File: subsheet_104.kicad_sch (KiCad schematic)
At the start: 0 parts

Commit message: almost done dma controller and acsi port
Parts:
- added C7: 0.1uF, commons-passives_THT:Passive_THT_capacitor_mlcc_W2.54mm_L12.70mm, symbol Device:C_Small
- added J2: DB19S ACSI, symbol Connector_Generic_Shielded:Conn_01x19_Shielded
- added L24: Ferrite bead, commons-passives_THT:Passive_THT_ferrite_bead_W3.81mm_L15.24mm, symbol Device:Ferrite_Bead_Small
- added R103: 1K, symbol Device:R_Small_US
- added U1: ST_DMA_DIP40_PHY, Package_DIP:DIP-40_W15.24mm_LongPads, symbol st_dma_dip40:ST_DMA_DIP40_PHY
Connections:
- new net +5V: L24.2, R103.2
- new net +5VP: C7.1, L24.1, U1.40 (VCC)
- new net 8MHZ: U1.39 (CLK)
- new net A1: U1.2 (A1)
- new net ACK: J2.14 (Pin_14), U1.37 (~{ACK})
- new net ACSI_PORT_DRQ: J2.19 (Pin_19), R103.1
- new net ACSI_PORT_INT: J2.10 (Pin_10)
- new net CA1: J2.16 (Pin_16), U1.26 (CA1)
- new net CA2: U1.27 (CA2)
- new net CD0: J2.1 (Pin_1), U1.36 (CD0)
- new net CD1: J2.2 (Pin_2), U1.35 (CD1)
- new net CD2: J2.3 (Pin_3), U1.34 (CD2)
- new net CD3: J2.4 (Pin_4), U1.33 (CD3)
- new net CD4: J2.5 (Pin_5), U1.32 (CD4)
- new net CD5: J2.6 (Pin_6), U1.31 (CD5)
- new net CD6: J2.7 (Pin_7), U1.30 (CD6)
- new net CD7: J2.8 (Pin_8), U1.29 (CD7)
- new net CS: J2.9 (Pin_9), U1.24 (~{HDCS})
- new net D0: U1.4 (D0)
- new net D1: U1.5 (D1)
- new net D10: U1.14 (D10)
- new net D11: U1.15 (D11)
- new net D12: U1.16 (D12)
- new net D13: U1.17 (D13)
- new net D14: U1.18 (D14)
- new net D15: U1.19 (D15)
- new net D2: U1.6 (D2)
- new net D3: U1.7 (D3)
- new net D4: U1.8 (D4)
- new net D5: U1.9 (D5)
- new net D6: U1.10 (D6)
- new net D7: U1.11 (D7)
- new net D8: U1.12 (D8)
- new net D9: U1.13 (D9)
- new net DMA_FDCS: U1.22 (~{FDCS})
- new net DMA_FDRQ: U1.21 (FDRQ)
- new net DMA_RW: J2.18 (Pin_18), U1.25 (CR/~{W})
- new net GND: C7.2, J2.11 (Pin_11), J2.13 (Pin_13), J2.15 (Pin_15), J2.17 (Pin_17), J2.SH (Shield), U1.20 (GND), U1.28 (GND)
- new net XFCS: U1.3 (~{FCS})
- new net XRDY: U1.38 (RDY)
- new net XRESET: J2.12 (Pin_12)
- new net XRXW: U1.1 (R/~{W})
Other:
- note added: "A1"
- note added: "D0"
- note added: "D1"
- note added: "D2"
- note added: "D3"
- note added: "D4"
- note added: "D5"
- note added: "D6"
- note added: "D7"
- note added: "DRQ"
- note added: "INT"
- note added: "R /W"
- note added: "RESET"

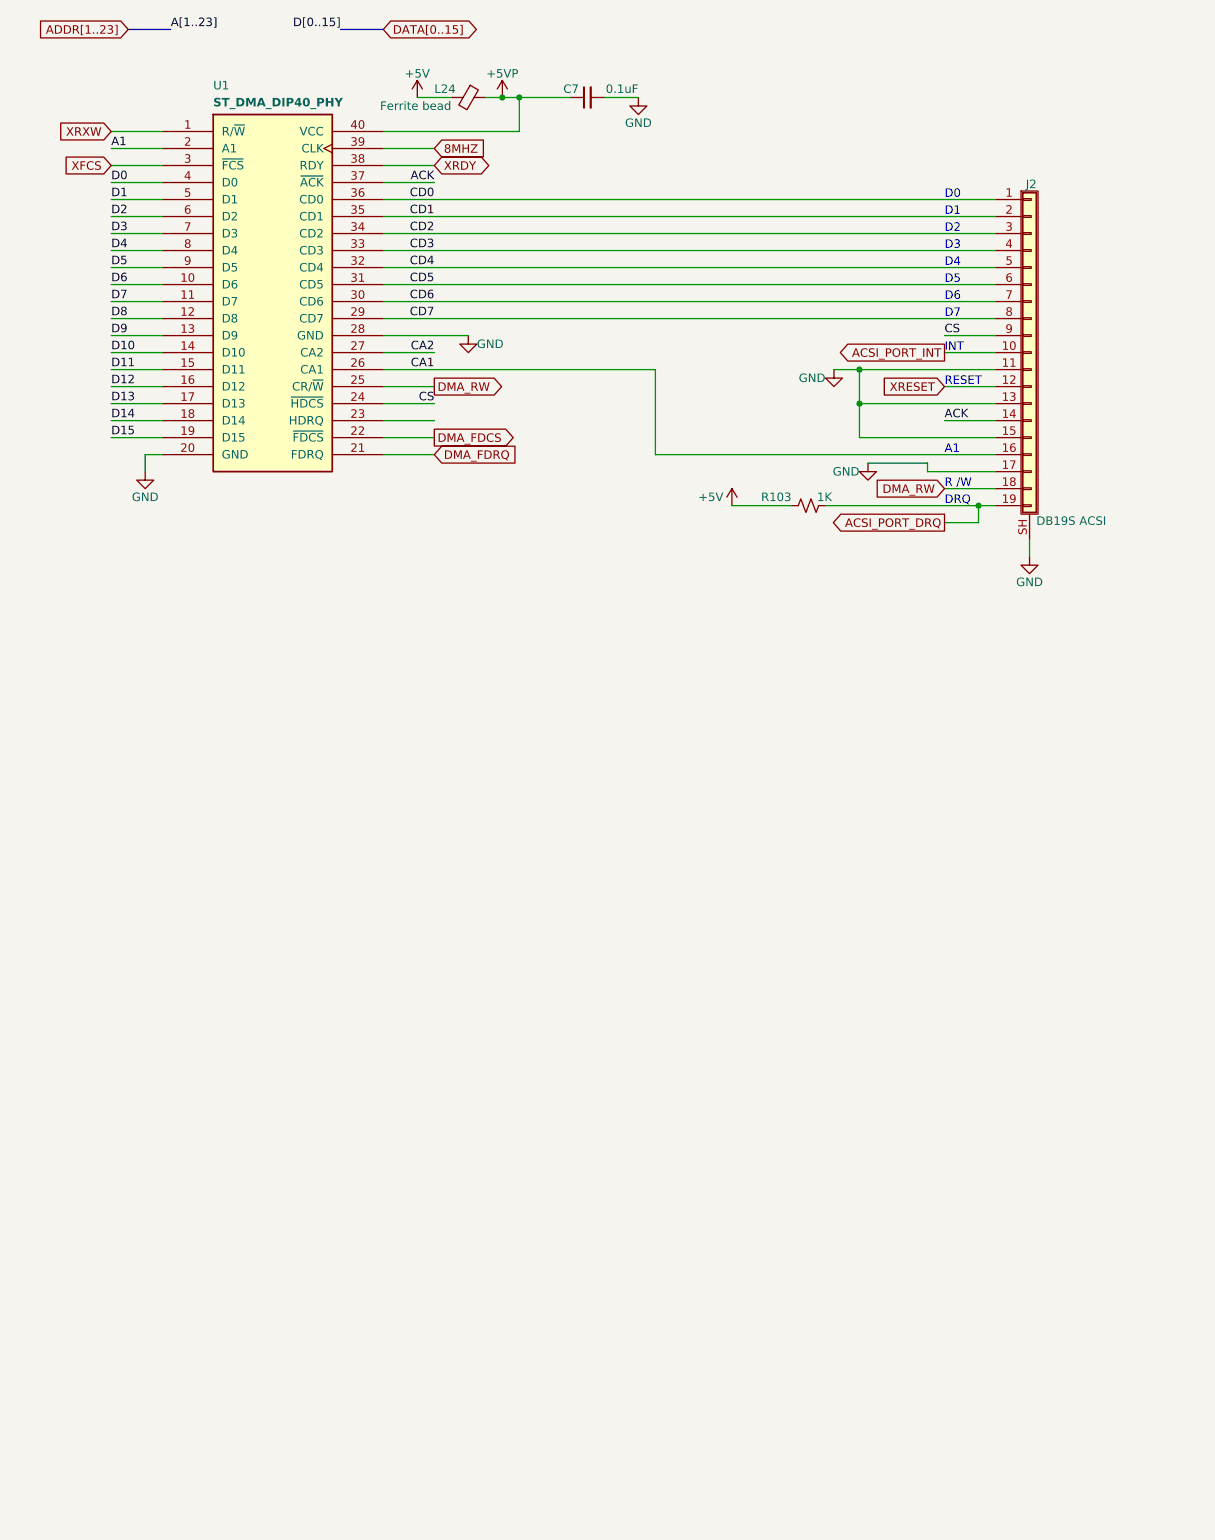
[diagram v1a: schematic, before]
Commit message: add floppy disk controller, port and 7406
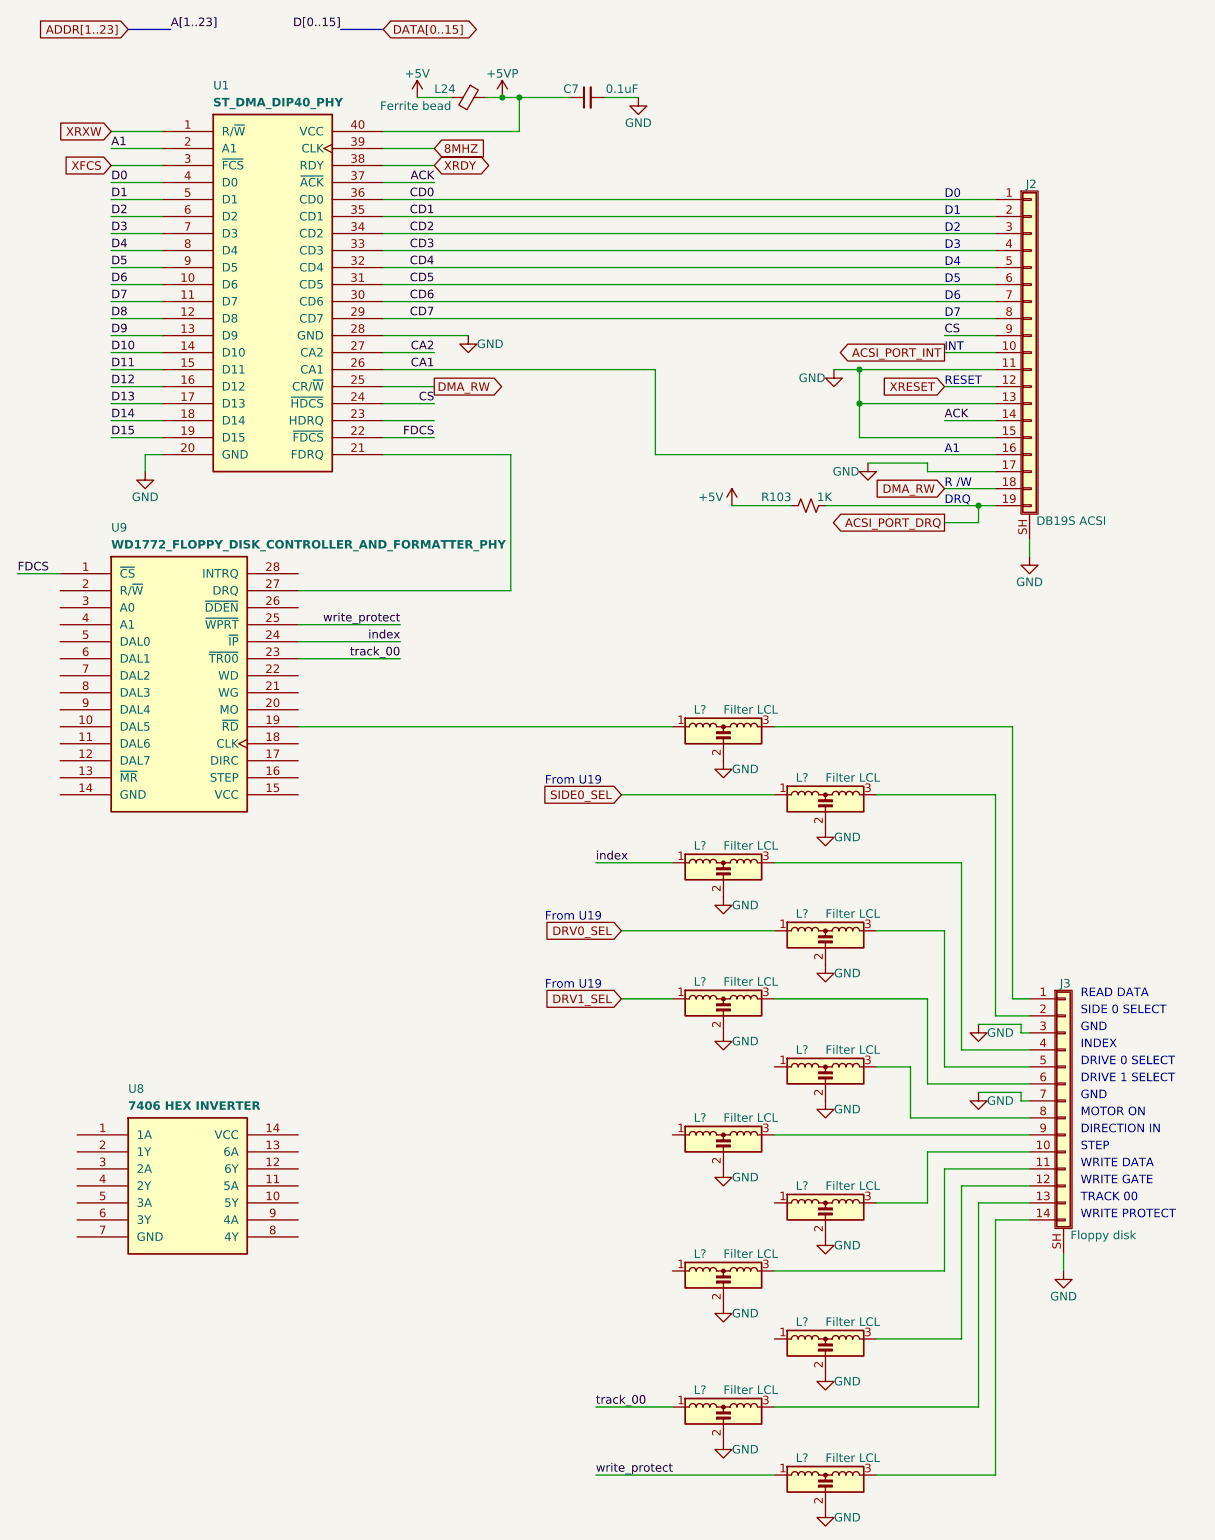
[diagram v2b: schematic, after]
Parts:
- added J3: Floppy disk, symbol Connector_Generic_Shielded:Conn_01x14_Shielded
- added L? (x12): Filter LCL, symbol Device:Filter_EMI_LCL
- added U8: 7406 HEX INVERTER, Package_DIP:DIP-14_W7.62mm_LongPads, symbol 74x06:74X06_HEX_INVERTER_BUFFERS_AND_DRIVERS_WITH_OPEN-COLLECTOR_HIGH-VOLTAGE_O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
- added U9: WD1772_FLOPPY_DISK_CONTROLLER_AND_FORMATTER_PHY, Package_DIP:DIP-28_W15.24mm_LongPads, symbol wd1772:WD1772_FLOPPY_DISK_CONTROLLER_AND_FORMATTER_PHY
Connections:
- net GND: now also J3.3 (Pin_3), J3.7 (Pin_7), J3.SH (Shield), L?.2, L?.2, L?.2, L?.2, L?.2, L?.2, L?.2, L?.2, L?.2, L?.2, L?.2, L?.2
- net DMA_FDCS renamed FDCS
- net FDCS: now also U9.1 (~{CS})
- net DMA_FDRQ: no longer names the net of U1.21 (FDRQ)
- net DMA_FDRQ: now also U9.27 (DRQ)
- new net: J3.9 (Pin_9), L?.3
- new net: J3.8 (Pin_8), L?.3
- new net: J3.1 (Pin_1), L?.3
- new net: J3.10 (Pin_10), L?.3
- new net: J3.11 (Pin_11), L?.3
- new net: J3.12 (Pin_12), L?.3
- new net: J3.13 (Pin_13), L?.3
- new net: J3.14 (Pin_14), L?.3
- new net: J3.2 (Pin_2), L?.3
- new net: J3.4 (Pin_4), L?.3
- new net: J3.5 (Pin_5), L?.3
- new net: J3.6 (Pin_6), L?.3
- new net: L?.1, U9.19 (~{RD})
- new net DRV0_SEL: L?.1
- new net DRV1_SEL: L?.1
- new net SIDE0_SEL: L?.1
- new net index: L?.1, U9.24 (~{IP})
- new net track_00: L?.1, U9.23 (~{TR00})
- new net write_protect: L?.1, U9.25 (~{WPRT})
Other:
- note added: "DIRECTION IN"
- note added: "DRIVE 0 SELECT"
- note added: "DRIVE 1 SELECT"
- note added: "From U19"
- note added: "GND"
- note added: "INDEX"
- note added: "MOTOR ON"
- note added: "READ DATA"
- note added: "SIDE 0 SELECT"
- note added: "STEP"
- note added: "TRACK 00"
- note added: "WRITE DATA"
- note added: "WRITE GATE"
- note added: "WRITE PROTECT"
